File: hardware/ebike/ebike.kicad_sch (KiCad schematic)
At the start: 19 parts, among them U1 STM32G431CBTx, Y1 ABLS-8MHZ-B2-T

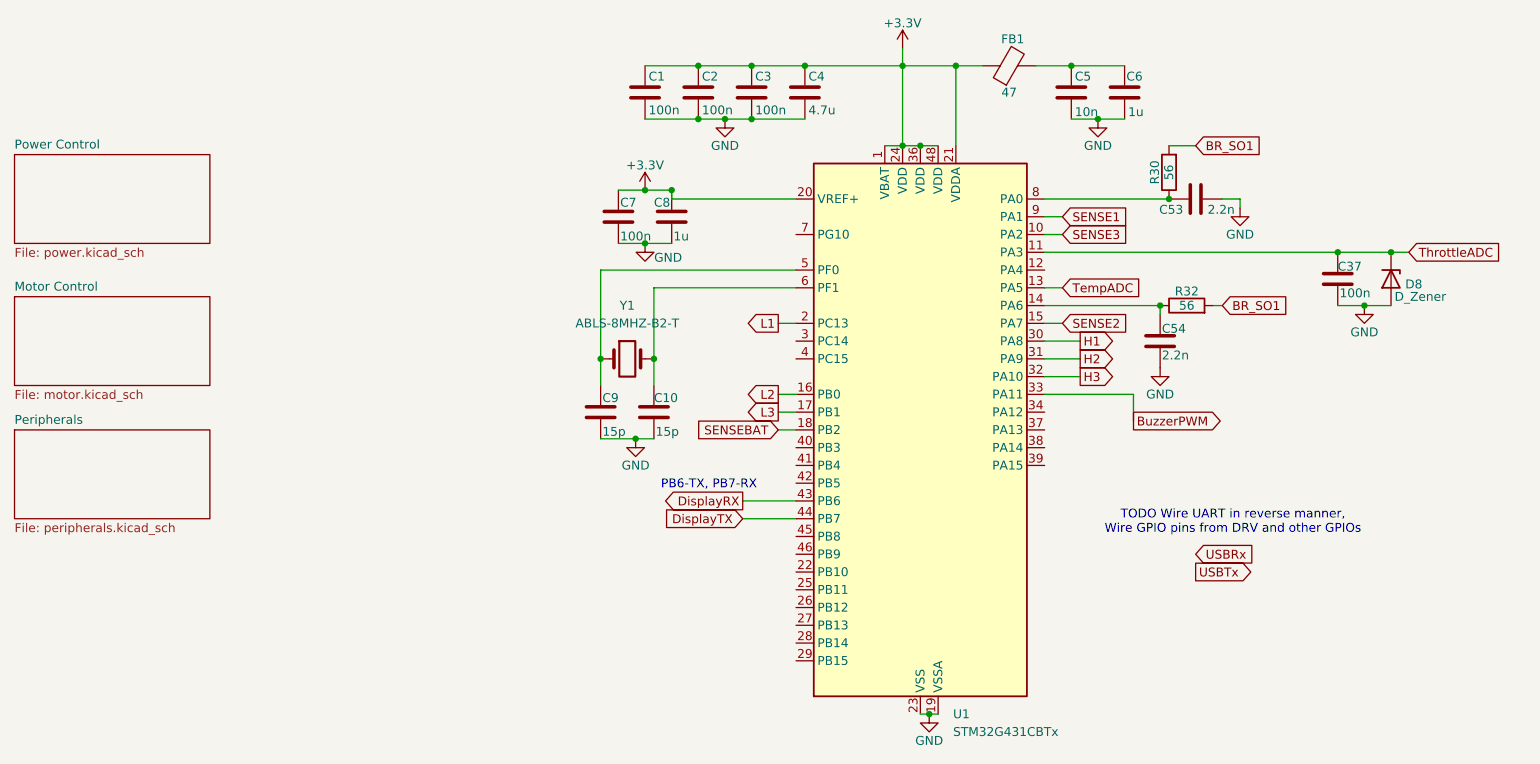
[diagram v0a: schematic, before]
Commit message: schematic ready for first review
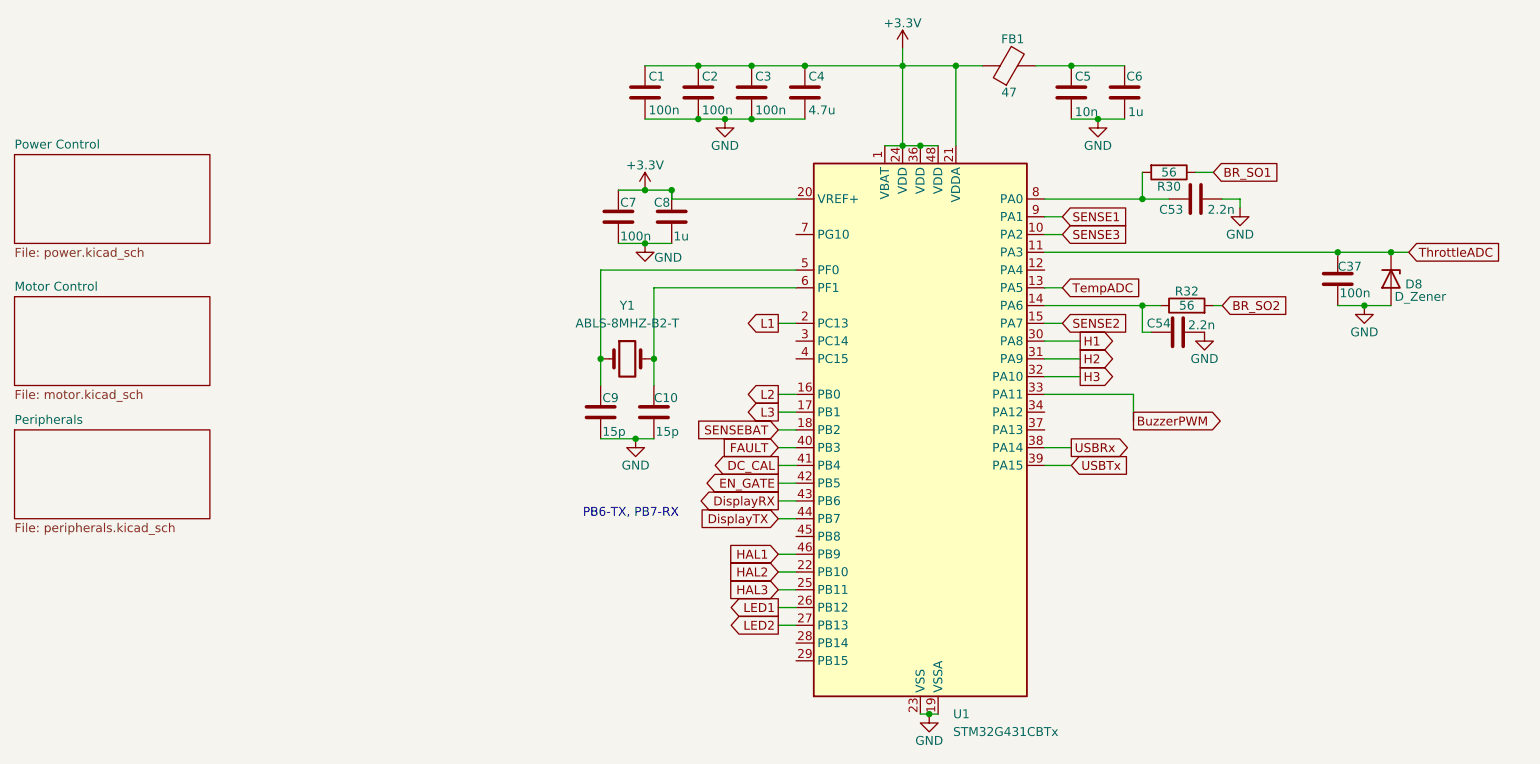
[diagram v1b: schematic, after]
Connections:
- net BR_SO1: now also R30.1; no longer R30.2, R32.2
- net USBRx: now also U1.38 (PA14)
- net USBTx: now also U1.39 (PA15)
- net at C53.1, U1.8 (PA0): now also R30.2; no longer R30.1
- net HAL2: now reaches U1.22 (PB10)
- net HAL3: now reaches U1.25 (PB11)
- net LED1: now reaches U1.26 (PB12)
- net LED2: now reaches U1.27 (PB13)
- net FAULT: now reaches U1.40 (PB3)
- net DC_CAL: now reaches U1.41 (PB4)
- net EN_GATE: now reaches U1.42 (PB5)
- net HAL1: now reaches U1.46 (PB9)
- new net BR_SO2: R32.2
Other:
- note removed: "TODO Wire UART in reverse manner, Wire GPIO pins from DRV and other GPIOs"
- moved on the sheet: C54, R30
